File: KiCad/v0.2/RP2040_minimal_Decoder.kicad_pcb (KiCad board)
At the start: 2 copper layers, 48.3 x 53.3 mm, 64 parts, among them J11 +V, J12 M_OUT_B, J13 M_OUT_A, J14 GND, J15 0, J16 1, J17 2, J18 3, J19 4, J2 Conn_01x02, J20 5, J21 SWCLK, J22 SWDIO, J23 RUN, J5 T0, J6 T1, J7 +3V3, Q1 T2N7002BK, Q2 T2N7002BK, Q3 T2N7002BK, Q4 T2N7002BK, Q5 T2N7002BK, U1 NCP1117-3.3_SOT223, U2 W25Q128JVS, U3 RP2040, U4 BDR6133, Y1 ABLS-12.000MHZ-B4-T

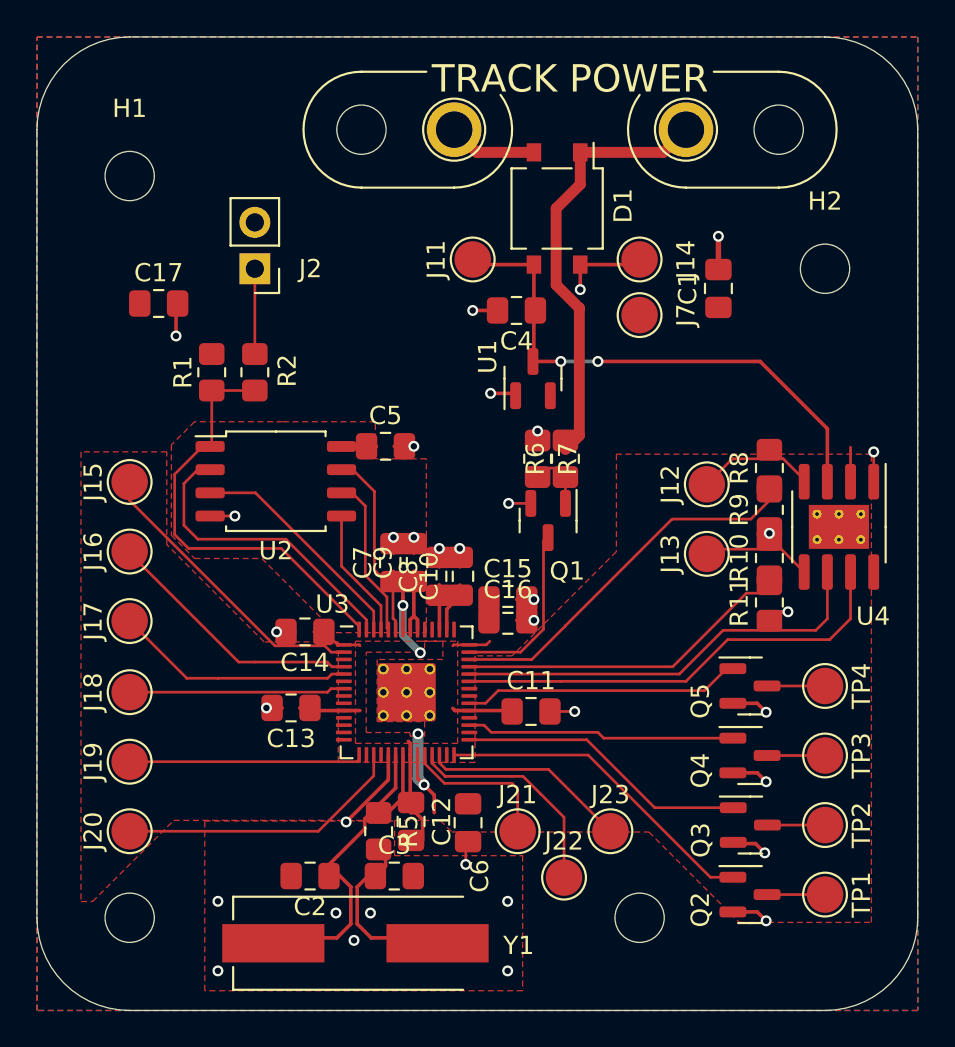
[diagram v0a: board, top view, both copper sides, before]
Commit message: cleaning up PCB
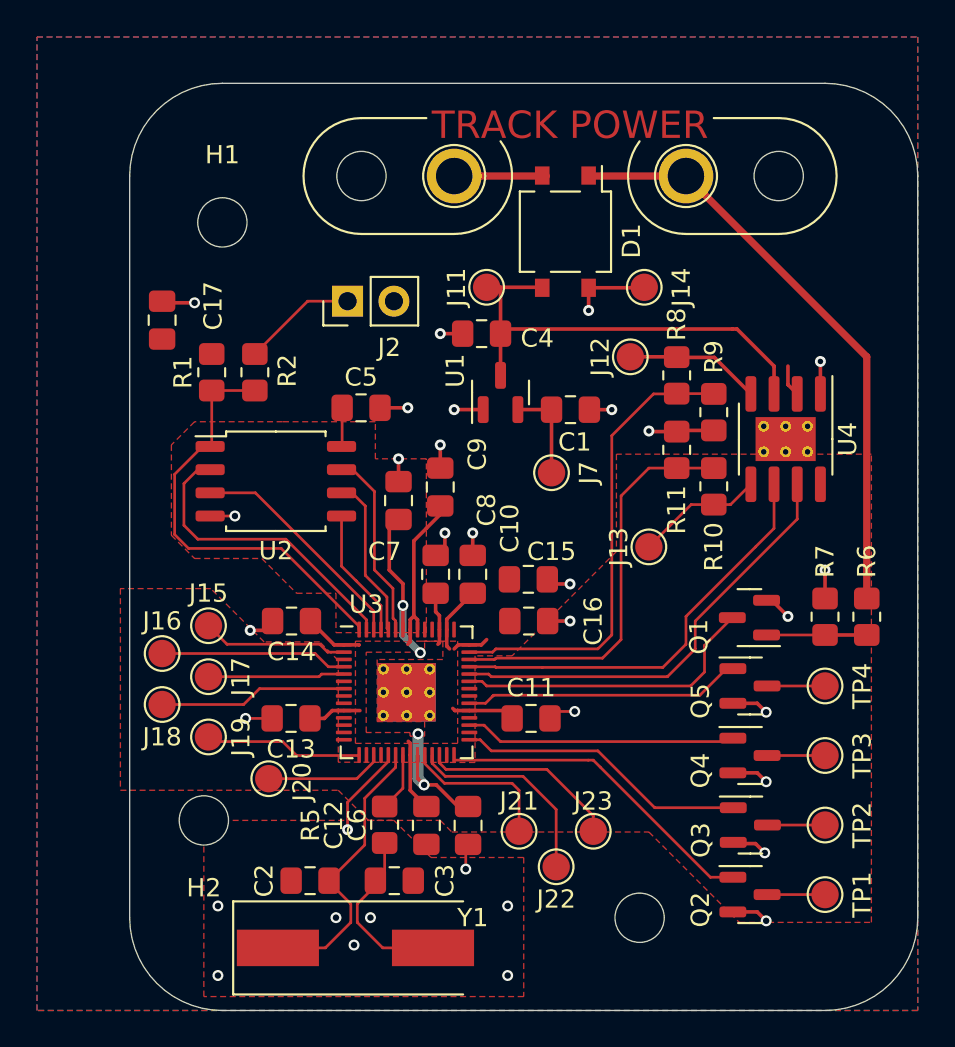
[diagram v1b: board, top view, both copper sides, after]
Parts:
- removed H4: MountingHole, MountingHole:MountingHole_2.7mm_M2.5
- J11, J12, J13, J14, J15, J16, J17, J18, J19, J20, J21, J22, J23, J7, TP1, TP2, TP3, TP4: footprint TestPoint:TestPoint_Pad_D2.0mm -> TestPoint:TestPoint_Pad_D1.5mm
- U3: footprint RP2040_minimal:RP2040-QFN-56 -> User:QFN-56-1EP_7x7mm_P0.4mm_EP3.2x3.2mm_BigThermalVias
- U4: footprint Package_SO:SOIC-8-1EP_3.9x4.9mm_P1.27mm_EP2.41x3.3mm_ThermalVias -> User:SOIC-8-1EP_3.9x4.9mm_P1.27mm_EP2.41x3.3mm_BigThermalVias
- Y1: footprint RP2040_minimal:Crystal_SMD_HC49-US -> Crystal:Crystal_SMD_HC49-SD
- moved H2 45.5 mm to (153.9, 111.5), turned to 180 degrees
- moved R6 18.6 mm to (190.2, 100.3)
- moved R7 18.0 mm to (188.0, 100.3)
- moved Q1 12.2 mm to (183.8, 100.4), turned to 180 degrees
- moved C1 10.5 mm to (174.0, 89.0), turned to 0 degrees
- moved J7 9.89 mm to (173.0, 92.5)
- moved R11 9.79 mm to (179.8, 91.2), turned to -90 degrees
- moved J15 8.98 mm to (154.2, 100.8), turned to 0 degrees
- moved J20 8.15 mm to (157.5, 109.2), turned to -90 degrees
- moved J12 8.15 mm to (177.3, 86.1)
- moved R8 7.18 mm to (179.8, 87.1)
- moved R9 6.16 mm to (181.9, 89.1)
- moved J16 5.86 mm to (151.6, 102.4), turned to 0 degrees
- moved H1 5.68 mm to (154.9, 78.7)
- moved U4 5.63 mm to (185.8, 90.6)
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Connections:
- U3 pad 37: /GPIO22 -> /GPIO21
- U3 pad 38: /GPIO23 -> /GPIO22
- U3 pad 39: /GPIO29_ADC3 -> /GPIO23
- U3 pad 40: /GPIO28_ADC2 -> /GPIO29_ADC3
- U3 pad 41: /GPIO21 -> /GPIO28_ADC2
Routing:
- net /GPIO5: track 15.8 -> 6.50 mm
- net +3V3: track 28.3 -> 37.5 mm
- net Net-(J5-Pin_1): track 24.0 -> 32.3 mm
- net /GPIO0: track 16.2 -> 8.02 mm
- net /GPIO21: track 9.68 -> 16.9 mm
- net /GPIO2: track 13.1 -> 7.48 mm
- net GND: track 42.4 -> 47.3 mm, vias 34 -> 33
- net +1V1: track 15.3 -> 20.1 mm
- net /GPIO28_ADC2: track 21.3 -> 25.7 mm
- net /GPIO4: track 12.9 -> 8.69 mm
- net VCC: track 29.4 -> 25.2 mm, vias 2 -> 0
- net /GPIO1: track 14.3 -> 10.3 mm
- net /GPIO29_ADC3: track 19.5 -> 22.3 mm
- net Net-(Q1-G): track 3.46 -> 5.49 mm
- net /~{USB_BOOT}: track 4.67 -> 6.28 mm
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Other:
- board size 48.3 x 53.3 mm -> 43.2 x 50.8 mm
